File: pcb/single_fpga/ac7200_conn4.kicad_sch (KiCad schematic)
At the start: 1 part, among them U97 ALINX AC7200 (XC7A200T-2FBG48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

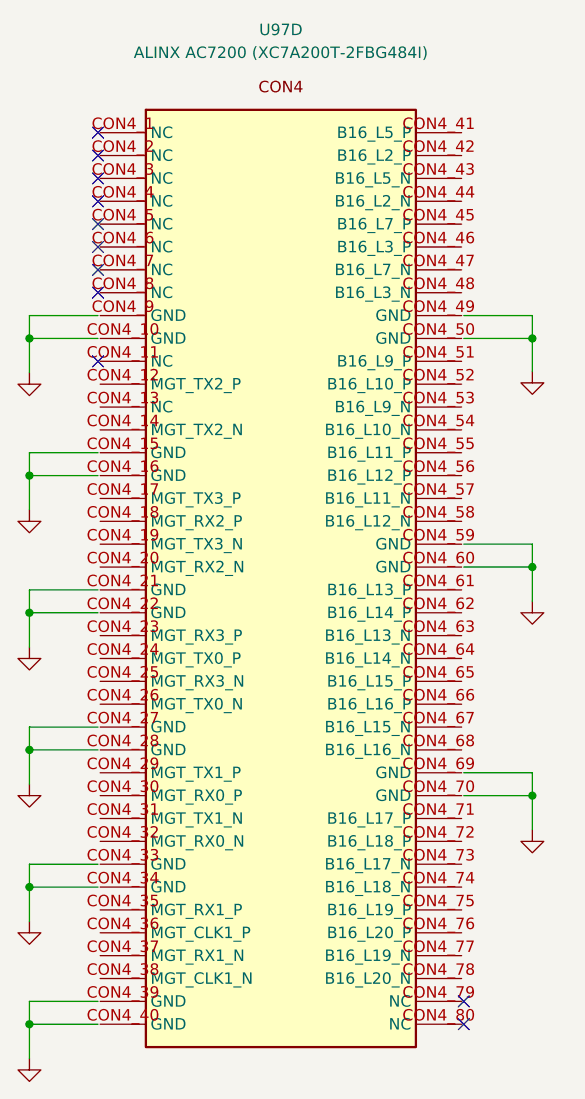
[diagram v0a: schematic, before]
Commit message: Changed position.
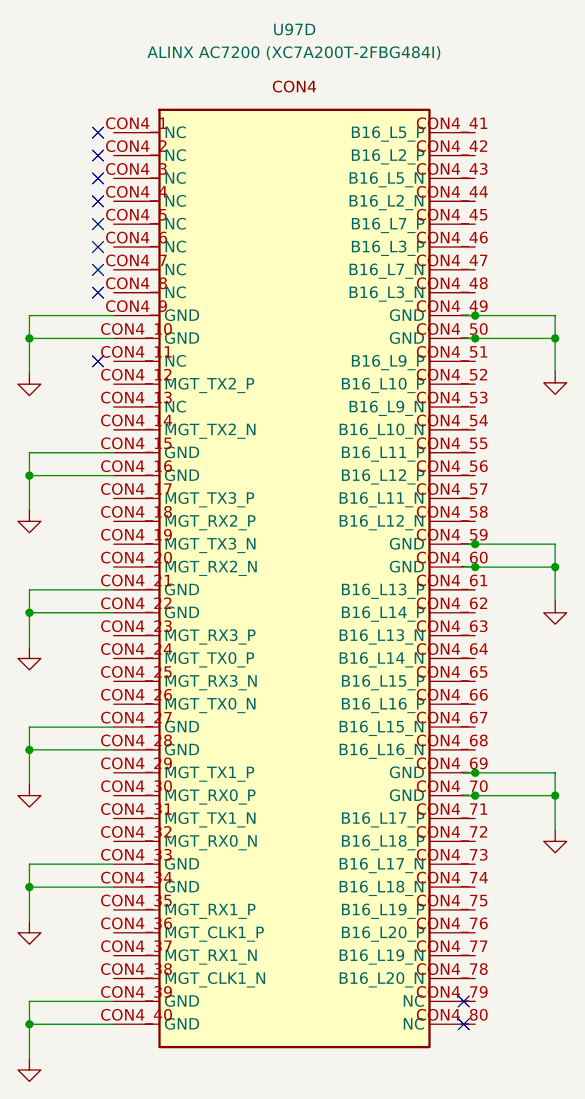
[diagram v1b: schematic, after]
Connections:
- net GND: now also U97.CON4_10 (GND), U97.CON4_15 (GND), U97.CON4_16 (GND), U97.CON4_21 (GND), U97.CON4_22 (GND), U97.CON4_27 (GND), U97.CON4_28 (GND), U97.CON4_33 (GND), U97.CON4_34 (GND), U97.CON4_39 (GND), U97.CON4_40 (GND), U97.CON4_49 (GND), U97.CON4_50 (GND), U97.CON4_59 (GND), U97.CON4_60 (GND), U97.CON4_69 (GND), U97.CON4_70 (GND), U97.CON4_9 (GND)
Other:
- moved on the sheet: U97D
